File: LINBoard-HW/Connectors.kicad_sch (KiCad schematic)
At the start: 5 parts, among them J2 TYPE-C 16PLT-H10.0, J4 ATM15-6P-BM03

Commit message: doing some layout
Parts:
- R13, R14: footprint Resistor_SMD:R_0402_1005Metric -> Resistor_SMD:R_0805_2012Metric
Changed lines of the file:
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@@
 			)
 		)
-		(property "Footprint" "Resistor_SMD:R_0402_1005Metric"
+		(property "Footprint" "Resistor_SMD:R_0805_2012Metric"
 			(at 96.52 153.67 0)
 			(effects
@@
 			)
 		)
-		(property "Footprint" "Resistor_SMD:R_0402_1005Metric"
+		(property "Footprint" "Resistor_SMD:R_0805_2012Metric"
 			(at 36.83 146.05 0)
 			(effects

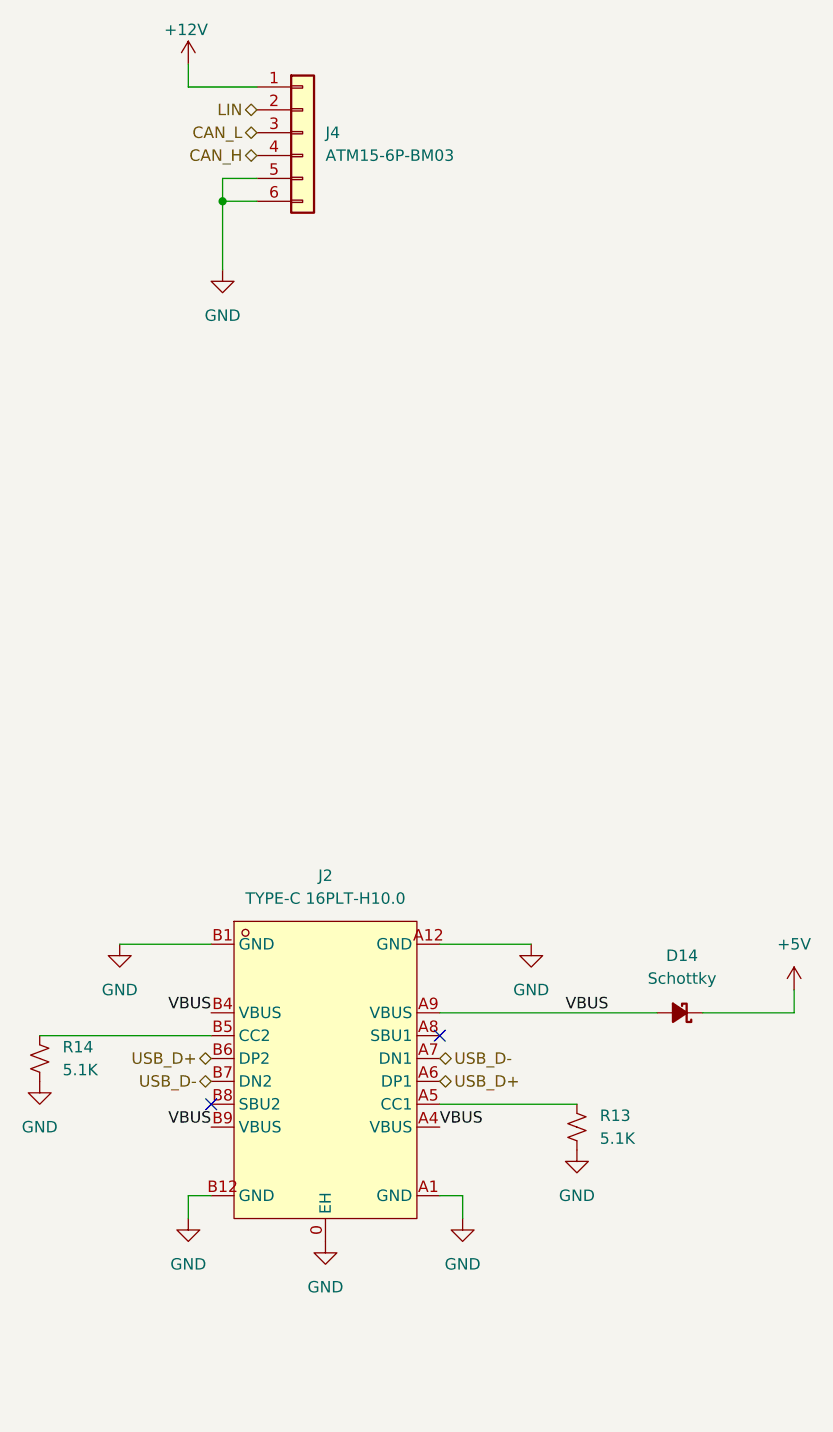
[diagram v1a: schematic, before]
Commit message: routing first pass complete
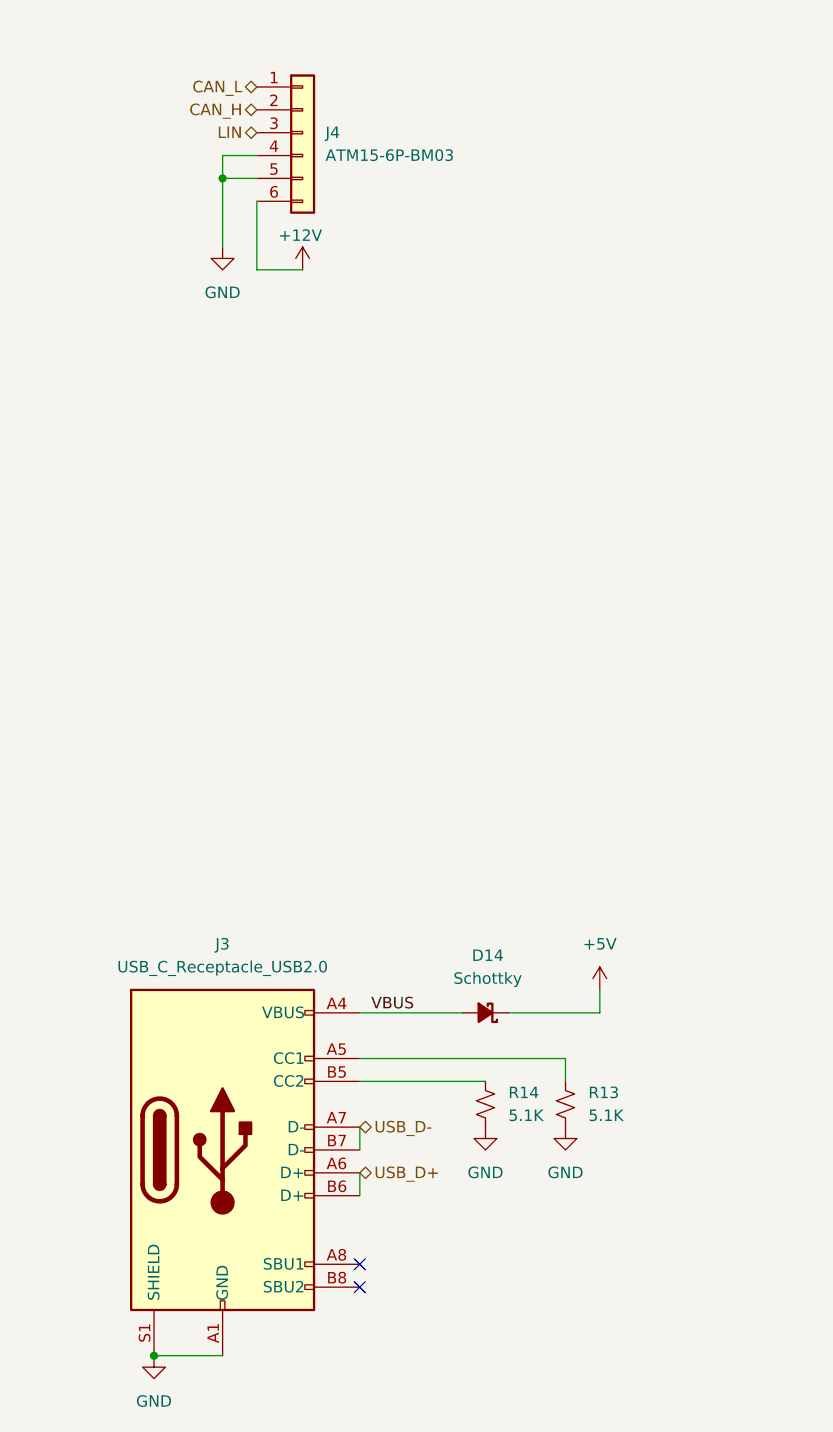
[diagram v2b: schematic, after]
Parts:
- removed J2: TYPE-C 16PLT-H10.0, Connector_USB:USB_C_Receptacle_GCT_USB4085, symbol vert_usb:TYPE-C16PLT-H10.0
- added J3: USB_C_Receptacle_USB2.0, Connector_USB:USB_C_Receptacle_GCT_USB4085, symbol Connectors:USB_C_Receptacle_USB2.0
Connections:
- net +12V: now also J4.6 (Pin_6); no longer J4.1 (Pin_1)
- net CAN_H: now also J4.2 (Pin_2); no longer J4.4 (Pin_4)
- net CAN_L: now also J4.1 (Pin_1); no longer J4.3 (Pin_3)
- net GND: now also J4.4 (Pin_4), J3.A1 (GND), J3.A12 (GND), J3.B1 (GND), J3.B12 (GND), J3.S1 (SHIELD); no longer J4.6 (Pin_6)
- net LIN: now also J4.3 (Pin_3); no longer J4.2 (Pin_2)
- net USB_D+: now also J3.A6 (D+), J3.B6 (D+)
- net USB_D-: now also J3.A7 (D-), J3.B7 (D-)
- net VBUS: now also J3.A4 (VBUS), J3.A9 (VBUS), J3.B4 (VBUS), J3.B9 (VBUS)
- net at R13.1: now also J3.A5 (CC1)
- net at R14.1: now also J3.B5 (CC2)
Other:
- moved on the sheet: D14, R13, R14
